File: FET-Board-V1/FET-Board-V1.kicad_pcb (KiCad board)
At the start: 2 copper layers, 100 x 100 mm, 167 parts, among them J201 STM32-Prog-Header, J301 USB_C_Receptacle_USB2.0_14P, J401 PHNX_CONN_1017521, J402 PHNX_CONN_1017521, J403 PHNX_CONN_1017521, J404 PHNX_CONN_1017521, Q1201 HCNR200-300E, Q401 BSC028N06LS3, Q402 BSC028N06LS3, Q403 BSC028N06LS3, Q404 BSC028N06LS3, Q405 BSC028N06LS3, Q406 BSC028N06LS3, Q407 BSC028N06LS3, Q501 HCNR200-300E, SW201 SW_Push, U1001 LTV-816S, U1002 LTC7001EMSE-TRPBF, U1101 LTV-816S, U1102 LTC7001EMSE-TRPBF, U1201 MCP6007, U1202 MCP6007, U1301 TPS259631, U1302 TPS259631, U1303 AZ1117IH-5.0, U1304 AZ1117IH-3.3, U201 MCP6007, U202 MCP6007, U203 MCP2542FD, U204 STM32G491KEUx, U301 USBLC6-2SC6, U401 LTV-816S, U501 MCP6007, U502 MCP6007, U601 ACS713xLCTR-30A, U701 ACS713xLCTR-30A, U801 ACS713xLCTR-30A, U901 LTV-816S, U902 LTC7001EMSE-TRPBF, X201 OXETDLJANF-8MHZ

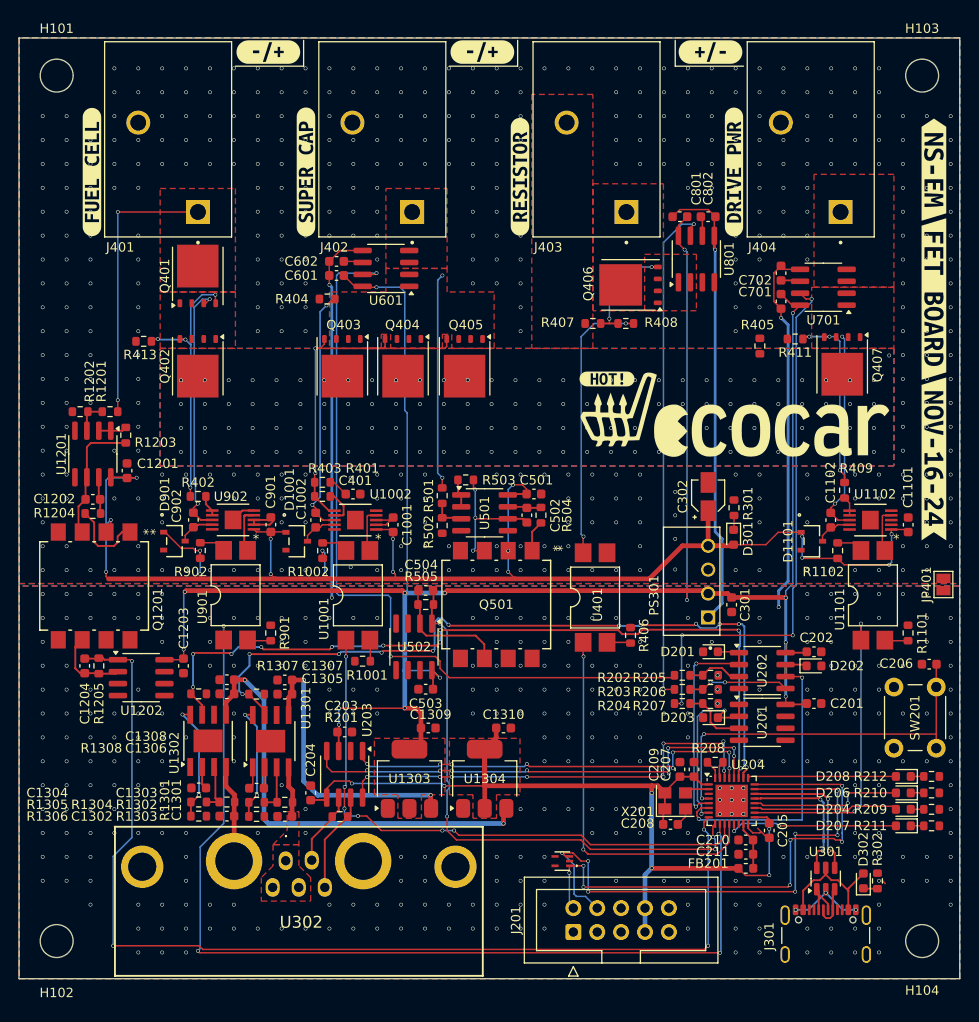
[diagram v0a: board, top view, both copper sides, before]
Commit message: update
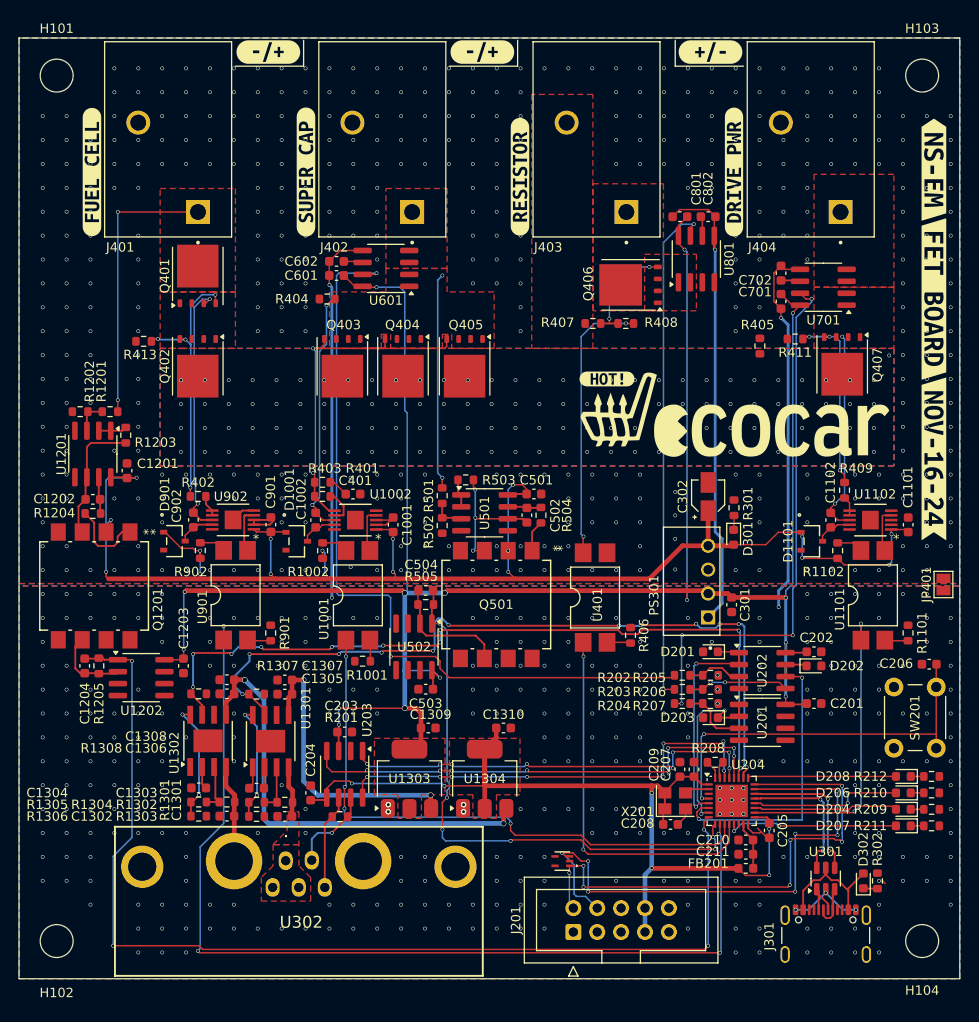
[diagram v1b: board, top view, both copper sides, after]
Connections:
- net /USB_HIGH_D+ renamed /High Power Controls/USB_HIGH_D+
- net /USB_HIGH_D- renamed /High Power Controls/USB_HIGH_D-
- R201 pad 1: /CAN_H_LOW -> /High Power Controls/CAN_H
- R201 pad 2: /CAN_H_HIGH -> /High Power Controls/CAN_L
- U203 pad 6: /CAN_H_HIGH -> /High Power Controls/CAN_L
- U203 pad 7: /CAN_H_LOW -> /High Power Controls/CAN_H
- U302 pad 2: /CAN_H_HIGH -> /High Power Controls/CAN_H
- U302 pad 5: /CAN_H_LOW -> /High Power Controls/CAN_L
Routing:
- net /CAN_H_LOW: track 10.7 -> 0.00 mm
- net /High Power Controls/CAN_L: track 0.00 -> 10.4 mm
- net /High Power Controls/CAN_H: track 0.00 -> 9.25 mm, vias 0 -> 1
- net /CAN_H_HIGH: track 8.05 -> 0.00 mm
- net /FET_SIGS_LS.VOLT_CAP_SENSE: track 59.3 -> 60.5 mm, vias 4 -> 6
- net /High Power Controls/Mains & FETS/FET Drive 2/TGDN: track 38.1 -> 38.8 mm
- net /FET_SIGS_LS.CNTRL_2: track 62.1 -> 62.7 mm, vias 6 -> 4
- net /Low Power Controls/PB3: track 81.7 -> 82.2 mm
- net GNDA: vias 314 -> 318
